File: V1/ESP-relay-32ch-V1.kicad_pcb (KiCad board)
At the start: 2 copper layers, 186 x 67.8 mm, 450 parts, among them J1 Conn_01x08, J10 USB, J11 ETHERNET, J2 Conn_01x08, J3 Conn_01x08, J4 Conn_01x08, J5 Conn_01x08, J6 Conn_01x08, J7 Conn_01x08, J8 Conn_01x08, J9 VIN, Q1 WPM2015-3/TR, Q10 MMBT2222A/SOT-23-3, Q11 MMBT2222A/SOT-23-3, Q12 MMBT2222A/SOT-23-3, Q13 MMBT2222A/SOT-23-3, Q14 MMBT2222A/SOT-23-3, Q15 MMBT2222A/SOT-23-3, Q16 MMBT2222A/SOT-23-3, Q17 MMBT2222A/SOT-23-3, Q18 MMBT2222A/SOT-23-3, Q19 MMBT2222A/SOT-23-3, Q2 LMUN2211LT1G, Q20 MMBT2222A/SOT-23-3, Q21 MMBT2222A/SOT-23-3, Q22 MMBT2222A/SOT-23-3, Q23 MMBT2222A/SOT-23-3, Q24 MMBT2222A/SOT-23-3, Q25 MMBT2222A/SOT-23-3, Q26 MMBT2222A/SOT-23-3, Q27 MMBT2222A/SOT-23-3, Q28 MMBT2222A/SOT-23-3, Q29 MMBT2222A/SOT-23-3, Q3 UMH3N, Q30 MMBT2222A/SOT-23-3, Q31 MMBT2222A/SOT-23-3, Q32 MMBT2222A/SOT-23-3, Q33 MMBT2222A/SOT-23-3, Q34 MMBT2222A/SOT-23-3, Q35 MMBT2222A/SOT-23-3, Q4 MMBT2222A/SOT-23-3, Q5 MMBT2222A/SOT-23-3, Q6 MMBT2222A/SOT-23-3, Q7 MMBT2222A/SOT-23-3, Q8 MMBT2222A/SOT-23-3, Q9 MMBT2222A/SOT-23-3, SW1 RESET, U1 SY8089A1AAC, U10 OR-3H4-4, U11 OR-3H4-4, U12 OR-3H4-4, U13 OR-3H4-4, U14 OR-3H4-4, U15 OR-3H4-4, U16 OR-3H4-4, U17 OR-3H4-4, U2 TX4138, U3 CH340C, U4 ESP32-WROOM-32E-8MB, U5 LAN8710A, U6 MCP23017_SS, U7 MCP23017_SS, U8 MCP23017_SS, U9 MCP23017_SS

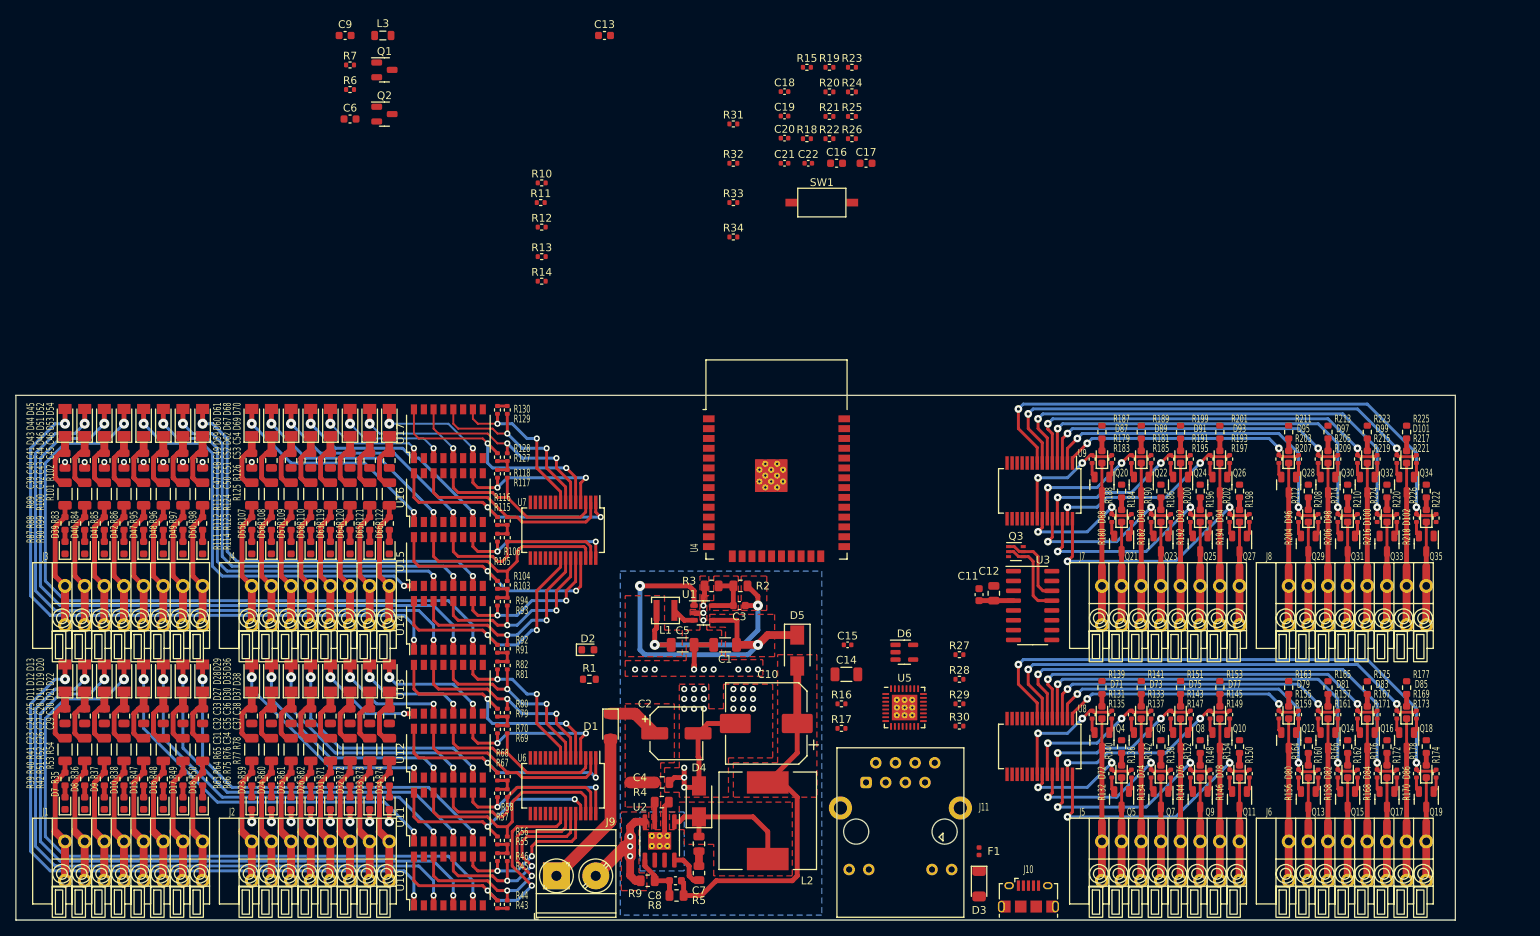
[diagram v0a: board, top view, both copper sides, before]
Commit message: Dev
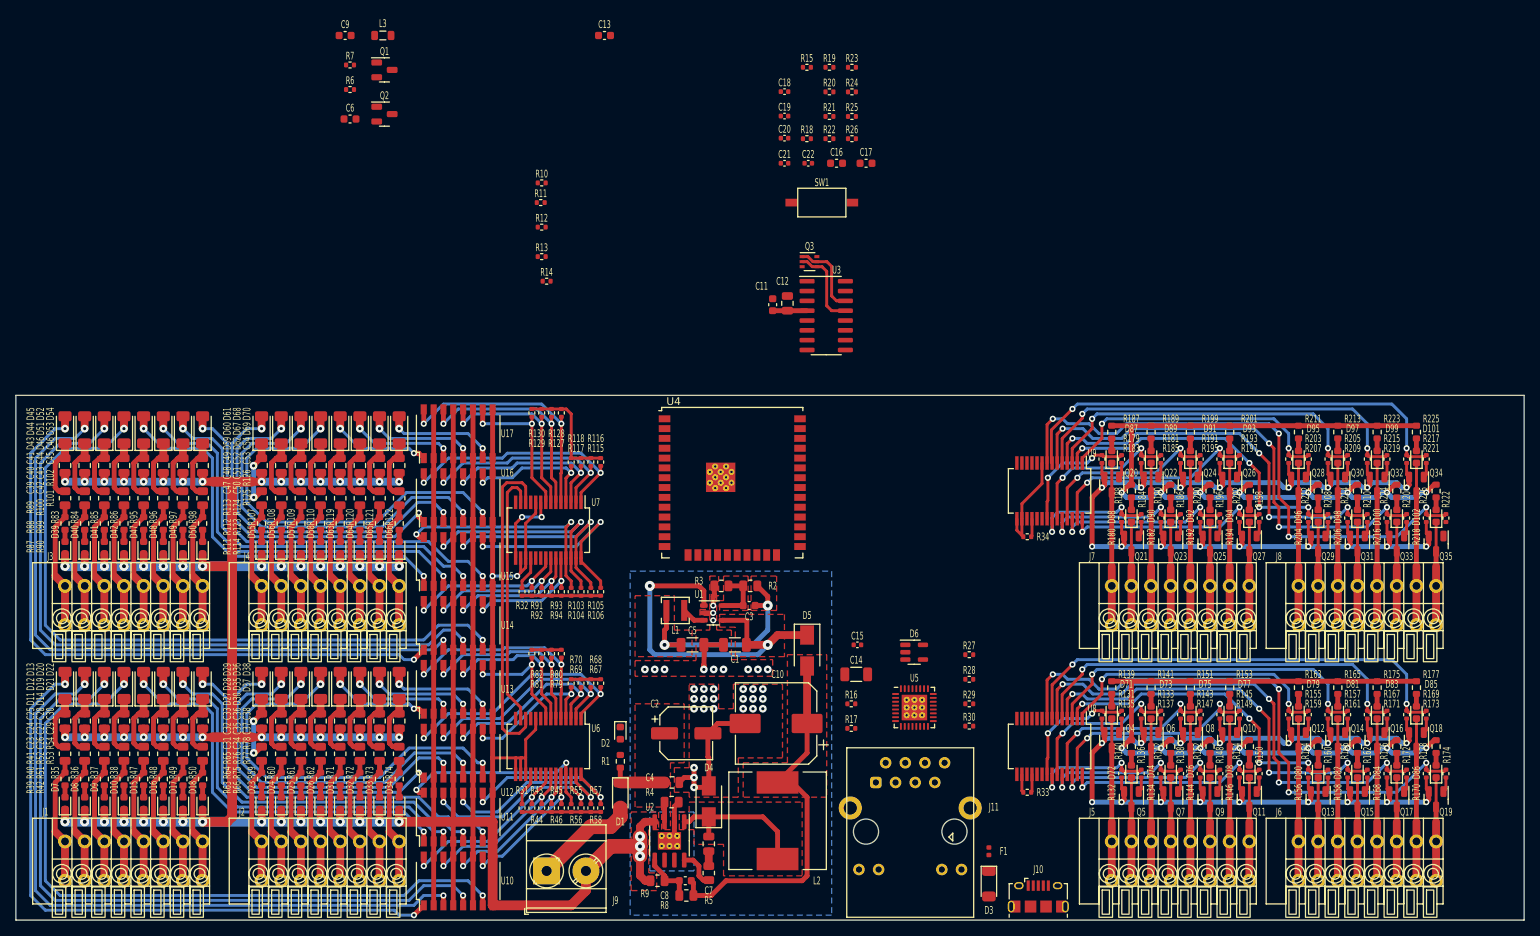
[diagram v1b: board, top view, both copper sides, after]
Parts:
- D10, D100, D101, D102, D15, D16, D17, D18, D2, D23, D24, D25, D26, D31, D32, D33, D34, D39, D40, D41, D42, D47, D48, D49, D50, D55, D56, D57, D58, D63, D64, D65, D66, D7, D71, D72, D73, D74, D75, D76, D77, D78, D79, D8, D80, D81, D82, D83, D84, D85, D86, D87, D88, D89, D9, D90, D91, D92, D93, D94, D95, D96, D97, D98, D99: value BLUE/0603 -> GREEN/0603
- D11, D12, D13, D14, D19, D20, D21, D22, D27, D28, D29, D30, D35, D36, D37, D38, D43, D44, D45, D46, D51, D52, D53, D54, D59, D60, D61, D62, D67, D68, D69, D70: footprint Tales:D_MiniMELF -> Diode_SMD:D_MiniMELF
- R100, R101, R102, R111, R112, R113, R114, R123, R124, R125, R126, R39, R40, R41, R42, R51, R52, R53, R54, R63, R64, R65, R66, R75, R76, R77, R78, R87, R88, R89, R90, R99: value 1k2/0,250W/1206 -> 1k8/0,125W/0805; footprint Tales:R_1206_3216Metric -> Tales:R_0805_2012Metric
- R103, R104, R105, R106, R115, R116, R117, R118, R127, R128, R129, R13, R130, R14, R15, R18, R19, R20, R21, R22, R23, R25, R43, R44, R45, R46, R55, R56, R57, R58, R67, R68, R69, R70, R79, R80, R81, R82, R91, R92, R93, R94: value 3k3/62,5mW/0402 -> 2k2/62,5mW/0402
- U4: value ESP32-WROOM-32E-8MB -> ESP32-WROOM-32UE-N16; footprint Tales:ESP32-WROOM-32 -> Tales:ESP32-WROOM-32U
- moved R31 92.5 mm to (130.2, 117.6), turned to 90 degrees
- moved R33 85.1 mm to (195.5, 115.6)
- moved R32 61.7 mm to (130.2, 89.7), turned to 90 degrees
- moved R34 54.2 mm to (195.5, 82.5)
- moved Q3 46.0 mm to (167.3, 47.0)
- moved U3 46.0 mm to (169.5, 54.0)
- moved C11 46.0 mm to (162.6, 52.6)
- moved C12 46.0 mm to (164.5, 52.4)
- moved R67 18.0 mm to (140.3, 101.5), turned to -90 degrees
- moved R68 16.2 mm to (139.1, 101.5), turned to -90 degrees
- moved R115 15.4 mm to (140.3, 72.9), turned to -90 degrees
- moved R106 15.1 mm to (140.3, 89.7), turned to 90 degrees
- moved R58 13.5 mm to (140.3, 117.6), turned to 90 degrees
- moved R43 13.2 mm to (131.4, 117.6)
- moved R44 13.2 mm to (132.7, 117.6)
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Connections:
- C21 pad 1: (no net) -> Net-(U5-VDDCR)
- C22 pad 1: (no net) -> Net-(U5-VDDCR)
- U5 pad 6: (no net) -> Net-(U5-VDDCR)
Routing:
- net GND: track 125.0 -> 973.6 mm, vias 53 -> 136
- net +24V: track 12.5 -> 217.3 mm, vias 0 -> 16
- net /MCU/I2C_SCL: track 0.00 -> 41.4 mm
- net +3.3V: track 61.4 -> 101.6 mm, vias 2 -> 4
- net /MCU/I2C_SDA: track 0.00 -> 33.6 mm
- net Net-(D62-A): track 28.9 -> 53.8 mm
- net Net-(D30-A): track 31.8 -> 54.2 mm
- net Net-(D61-A): track 28.9 -> 50.8 mm
- net Net-(D29-A): track 31.1 -> 51.2 mm
- net Net-(D60-A): track 28.9 -> 47.7 mm
- net Net-(D28-A): track 30.4 -> 48.1 mm
- net Net-(D59-A): track 28.9 -> 43.6 mm
- net /GPIO Expanders/IN1: track 37.9 -> 23.5 mm
- net Net-(D27-A): track 29.6 -> 42.9 mm
- net /GPIO Expanders/IN17: track 33.2 -> 21.4 mm
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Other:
- board size 186 x 67.8 mm -> 194.9 x 67.8 mm
